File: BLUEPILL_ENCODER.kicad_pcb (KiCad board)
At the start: 2 copper layers, 24.4 x 22 mm, 29 parts, among them J1 boot, J2 Conn_01x04, J3 USB_C_Receptacle_USB2.0_16P, J4 Conn_01x08, SW1 RESET_SWITCH, U1 STM32F103C8T6, U2 AMS1117-3.3, U4 AS5600L-ASOM, Y2 8Mz

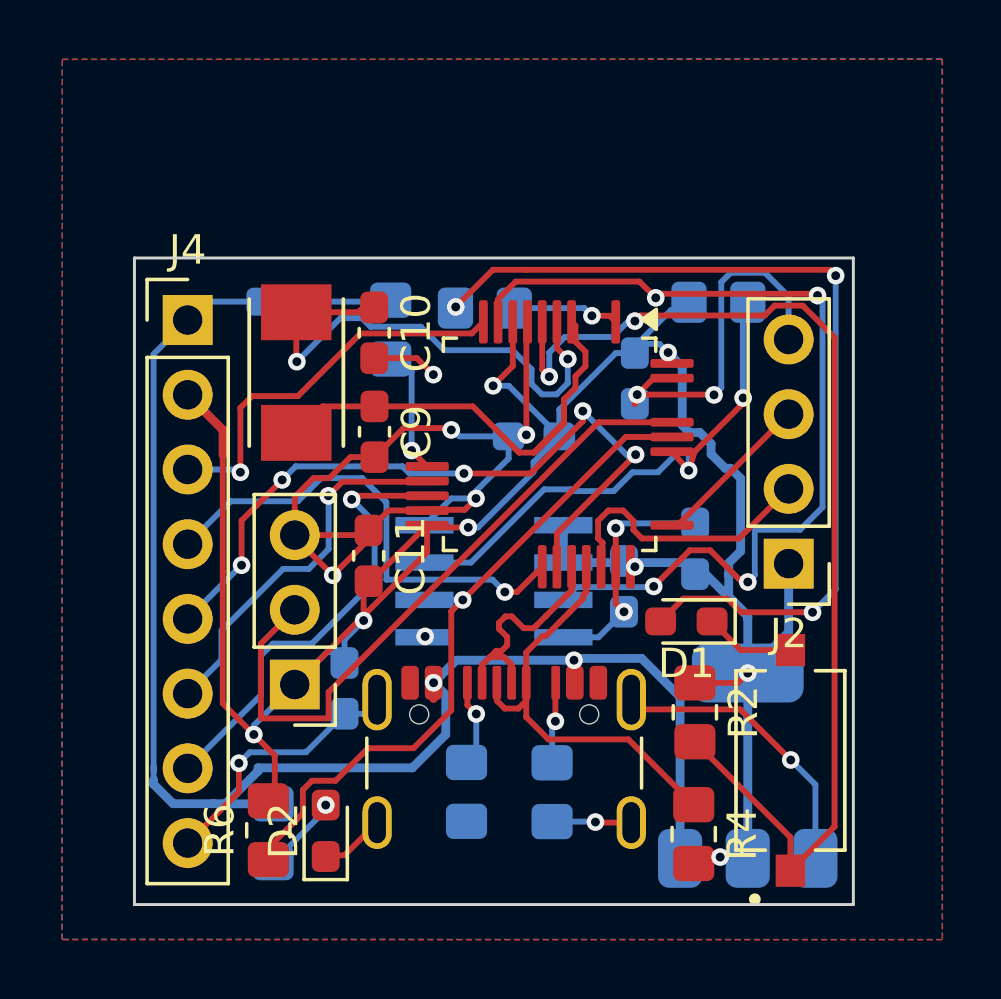
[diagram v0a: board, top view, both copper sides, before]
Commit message: Add files via upload
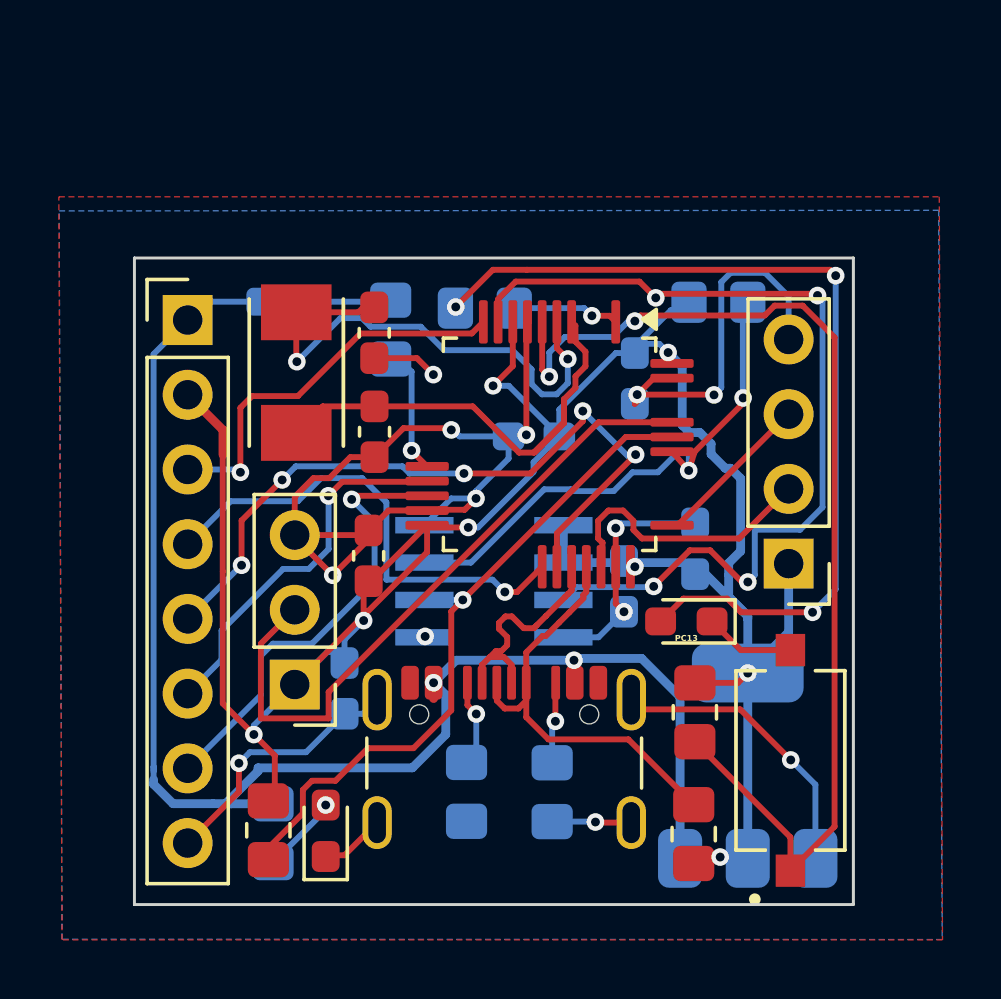
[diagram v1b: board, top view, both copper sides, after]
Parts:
- renumbered D1 to PC13
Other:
- board text added: "PC13"
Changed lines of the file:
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@@
 			(at 0 -2.38 0)
 			(layer "F.SilkS")
+			(hide yes)
 			(effects
 				(font
@@
 			(at 0 -1.43 270)
 			(layer "F.SilkS")
+			(hide yes)
 			(effects
 				(font
@@
 		(descr "LED SMD 0603 (1608 Metric), square (rectangular) end terminal, IPC-7351 nominal, (Body size source: http://www.tortai-tech.com/upload/download/2011102023233369053.pdf), generated with kicad-footprint-generator")
 		(tags "LED handsolder")
-		(property "Reference" "D1"
-			(at 0 -1.43 0)
+		(property "Reference" "PC13"
+			(at 0 -0.53 0)
 			(layer "F.SilkS")
+			(hide yes)
 			(effects
 				(font
-					(size 1 1)
-					(thickness 0.15)
+					(size 0.2 0.2)
+					(thickness 0.05)
+					(bold yes)
 				)
 			)
@@
 			(layer "F.Fab")
 		)
-		(fp_text user "${REFERENCE}"
-			(at 0 0 0)
-			(layer "F.Fab")
-			(effects
-				(font
-					(size 0.4 0.4)
-					(thickness 0.06)
-				)
-			)
-		)
 		(pad "1" smd roundrect
 			(at -0.875 0 180)
@@
 			(at 14.64 -0.32 0)
 			(layer "F.Fab")
+			(hide yes)
 			(effects
 				(font
@@
 			(layer "F.Fab")
 		)
-		(fp_text user "${REFERENCE}"
-			(at 11.5 -1.37 90)
-			(layer "F.Fab")
-			(effects
-				(font
-					(size 1 1)
-					(thickness 0.15)
-				)
-			)
-		)
 		(pad "1" thru_hole rect
 			(at 0 0 180)
@@
 			(at 0 -1.43 270)
 			(layer "F.SilkS")
+			(hide yes)
 			(effects
 				(font
@@
 			(at 0 -1.65 90)
 			(layer "F.SilkS")
+			(hide yes)
 			(effects
 				(font
@@
 			(at 0 -2.38 0)
 			(layer "F.SilkS")
+			(hide yes)
 			(effects
 				(font
@@
 			(at 0 -1.43 90)
 			(layer "F.SilkS")
+			(hide yes)
 			(effects
 				(font
@@
 			(at 0 -1.43 270)
 			(layer "F.SilkS")
+			(hide yes)
 			(effects
 				(font
@@
 			(at 0 -1.65 90)
 			(layer "F.SilkS")
+			(hide yes)
 			(effects
 				(font
@@
 			(at 0 -1.65 90)
 			(layer "F.SilkS")
+			(hide yes)
 			(effects
 				(font
@@
 			(at 0 1.65 90)
 			(layer "B.SilkS")
+			(hide yes)
 			(effects
 				(font
@@
 			(at 0 1.65 90)
 			(layer "B.SilkS")
+			(hide yes)
 			(effects
 				(font
@@
 			(at 0 1.65 0)
 			(layer "B.SilkS")
+			(hide yes)
 			(effects
 				(font
@@
 			(at 0 1.65 90)
 			(layer "B.SilkS")
+			(hide yes)
 			(effects
 				(font
@@
 			(at 0 1.43 0)
 			(layer "B.SilkS")
+			(hide yes)
 			(effects
 				(font
@@
 			(at 0 1.43 0)
 			(layer "B.SilkS")
+			(hide yes)
 			(effects
 				(font
@@
 			(unlocked yes)
 			(layer "B.SilkS")
+			(hide yes)
 			(effects
 				(font
@@
 			(at 0 1.43 90)
 			(layer "B.SilkS")
+			(hide yes)
 			(effects
 				(font
@@
 			(at 0 1.43 90)
 			(layer "B.SilkS")
+			(hide yes)
 			(effects
 				(font
@@
 			(at 0 1.65 0)
 			(layer "B.SilkS")
+			(hide yes)
 			(effects
 				(font
@@
 			(at 0 1.43 90)
 			(layer "B.SilkS")
+			(hide yes)
 			(effects
 				(font
@@
 			(at 0 1.43 270)
 			(layer "B.SilkS")
+			(hide yes)
 			(effects
 				(font
@@
 			(at 0 1.65 90)
 			(layer "B.SilkS")
+			(hide yes)
 			(effects
 				(font
@@
 		(layer "Edge.Cuts")
 	)
+	(gr_text "PC13"
+		(at 187.96 71.8 0)
+		(layer "F.SilkS")
+		(effects
+			(font
+				(size 0.2 0.2)
+				(thickness 0.05)
+				(bold yes)
+			)
+		)
+	)
 	(gr_text "PCB Edge"
 		(at 181.7678 80.095 0)
@@
 		(polygon
 			(pts
-				(xy 166.7378 52.125) (xy 196.6678 52.125) (xy 196.6678 82.055) (xy 166.7378 82.055)
+				(xy 166.6278 56.795) (xy 196.5578 56.795) (xy 196.6678 82.055) (xy 166.7378 82.055)
 			)
 		)
@@
 		(polygon
 			(pts
-				(xy 166.7478 52.125) (xy 196.6478 52.105) (xy 196.6578 82.045) (xy 166.7378 82.035)
+				(xy 166.6378 57.275) (xy 196.5378 57.255) (xy 196.6578 82.045) (xy 166.7378 82.035)
 			)
 		)

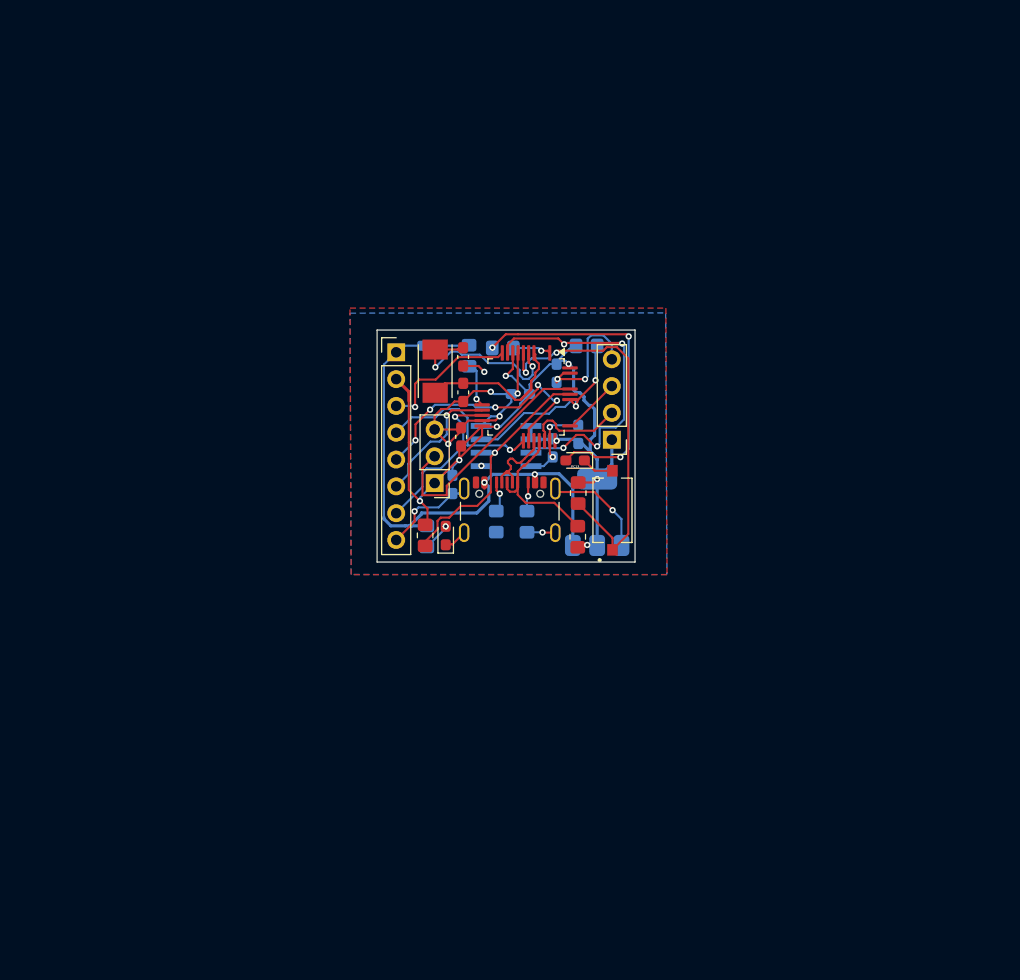
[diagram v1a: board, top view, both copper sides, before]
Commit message: Add files via upload
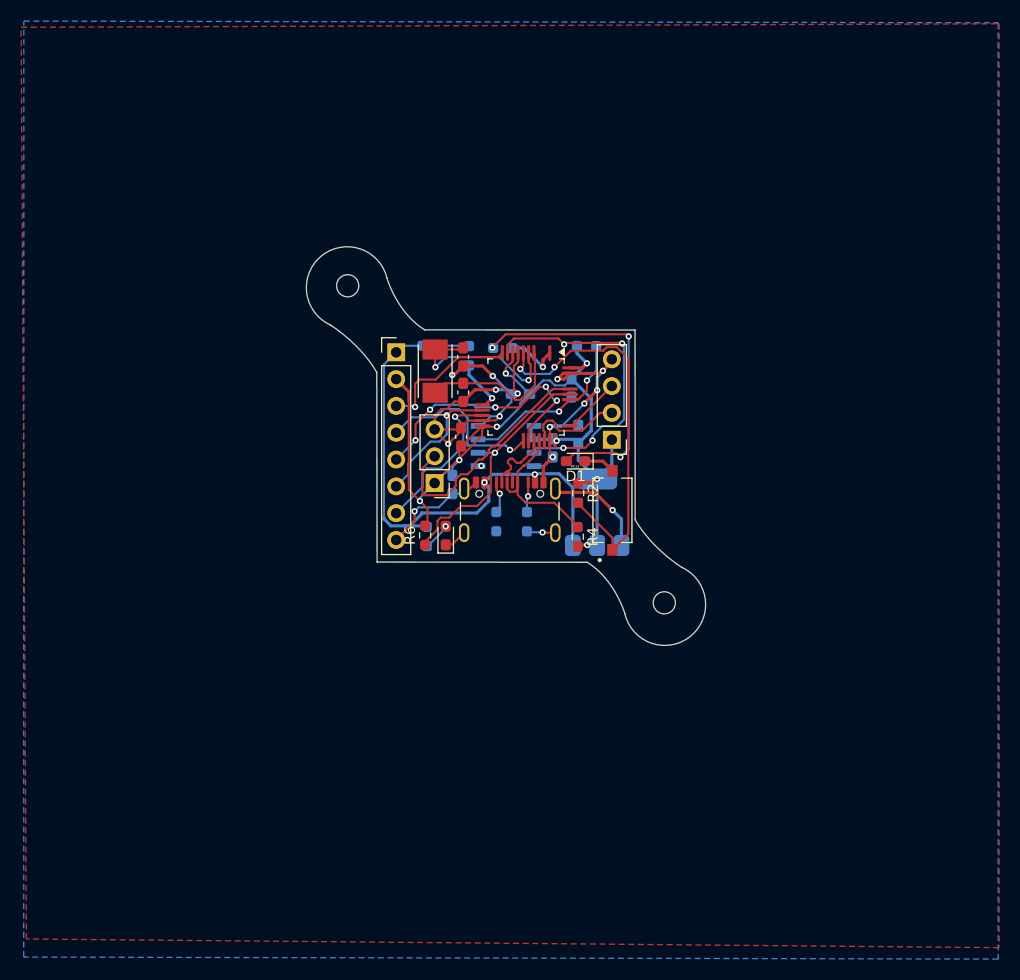
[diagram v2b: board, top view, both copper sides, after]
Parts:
- removed PC13: LED, LED_SMD:LED_0603_1608Metric_Pad1.05x0.95mm_HandSolder
- added D1: LED, LED_SMD:LED_0603_1608Metric_Pad1.05x0.95mm_HandSolder, F.Cu at (188.0, 71.3)
- added REF**: MountingHole_2.1mm, MountingHole:MountingHole_2.1mm, F.Cu at (166.4, 54.7)
- added REF**: MountingHole_2.1mm, MountingHole:MountingHole_2.1mm, F.Cu at (196.4, 84.7)
- R1, R2, R3, R4, R5, R6, R7, R8, R9: footprint Resistor_SMD:R_0805_2012Metric_Pad1.20x1.40mm_HandSolder -> Resistor_SMD:R_0603_1608Metric_Pad0.98x0.95mm_HandSolder
- U4: footprint AS5600:SOIC8_AS5600_OSR -> ul_AS5600L-ASOM:AS5600L-ASOM_AMS
- moved C3 1.98 mm to (187.6, 64.4)
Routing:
- net GND: track 82.5 -> 94.7 mm, vias 13 -> 16
- net HSE_IN: track 16.7 -> 14.1 mm
- net I2C_SCL: track 18.6 -> 16.6 mm
- net 3.3V_MAIN_POWER_RAIL: track 89.5 -> 87.6 mm
- net LED_BINK: track 3.64 -> 5.23 mm
- net SENSOR_ANLG_OUT: track 32.0 -> 30.4 mm
- net HSE_OUT: track 18.2 -> 17.3 mm
- net BOOT1: track 4.33 -> 5.14 mm
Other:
- board size 24.4 x 22 mm -> 37.8 x 37.8 mm
